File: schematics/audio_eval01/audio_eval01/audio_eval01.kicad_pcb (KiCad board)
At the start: 2 copper layers, 31.1 x 28.6 mm, 2 parts, among them J1 Conn_01x08_Pin

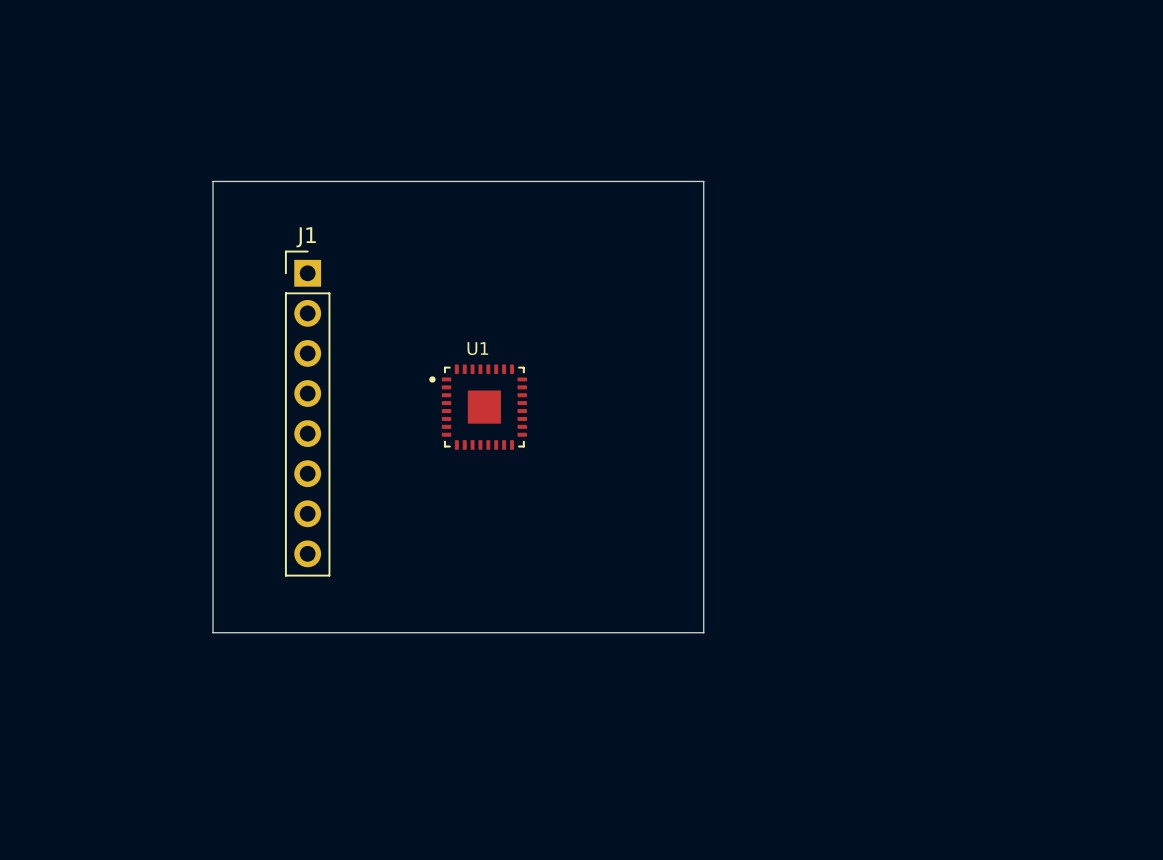
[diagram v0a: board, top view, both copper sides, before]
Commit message: Audio evaluation board work.
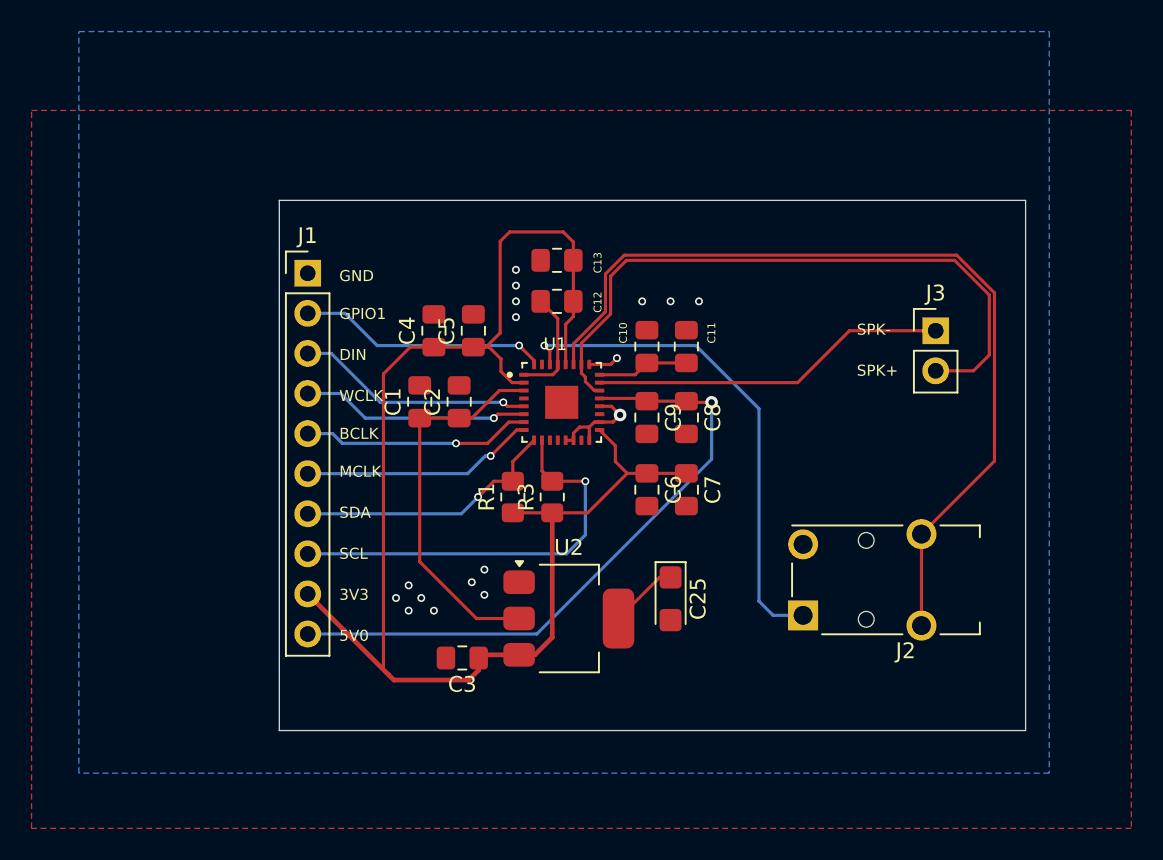
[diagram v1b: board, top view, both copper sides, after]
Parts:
- added C1: 0.1uF, Capacitor_SMD:C_0805_2012Metric_Pad1.18x1.45mm_HandSolder, F.Cu at (136.1, 83.0)
- added C10: 0.1uF, Capacitor_SMD:C_0805_2012Metric_Pad1.18x1.45mm_HandSolder, F.Cu at (150.5, 79.5)
- added C11: 22uF, Capacitor_SMD:C_0805_2012Metric_Pad1.18x1.45mm_HandSolder, F.Cu at (153.0, 79.5)
- added C12: 0.1uF, Capacitor_SMD:C_0805_2012Metric_Pad1.18x1.45mm_HandSolder, F.Cu at (144.8, 76.6)
- added C13: 10uF, Capacitor_SMD:C_0805_2012Metric_Pad1.18x1.45mm_HandSolder, F.Cu at (144.8, 74.0)
- added C2: 10uF, Capacitor_SMD:C_0805_2012Metric_Pad1.18x1.45mm_HandSolder, F.Cu at (138.6, 83.0)
- added C25: 47uF, Capacitor_Tantalum_SMD:CP_EIA-3216-18_Kemet-A, F.Cu at (152.0, 95.4)
- added C3: 10uF, Capacitor_SMD:C_0805_2012Metric_Pad1.18x1.45mm_HandSolder, F.Cu at (138.8, 99.2)
- added C4: 0.1uF, Capacitor_SMD:C_0805_2012Metric_Pad1.18x1.45mm_HandSolder, F.Cu at (137.0, 78.5)
- added C5: 10uF, Capacitor_SMD:C_0805_2012Metric_Pad1.18x1.45mm_HandSolder, F.Cu at (139.5, 78.5)
- added C6: 0.1uF, Capacitor_SMD:C_0805_2012Metric_Pad1.18x1.45mm_HandSolder, F.Cu at (150.5, 88.5)
- added C7: 10uF, Capacitor_SMD:C_0805_2012Metric_Pad1.18x1.45mm_HandSolder, F.Cu at (153.0, 88.5)
- added C8: 0.1uF, Capacitor_SMD:C_0805_2012Metric_Pad1.18x1.45mm_HandSolder, F.Cu at (153.0, 84.0)
- added C9: 22uF, Capacitor_SMD:C_0805_2012Metric_Pad1.18x1.45mm_HandSolder, F.Cu at (150.5, 84.0)
- added J2: AudioJack3, Connector_Audio:Jack_3.5mm_Switronic_ST-005-G_horizontal, F.Cu at (166.9, 94.2)
- added J3: Conn_01x02_Pin, Connector_PinHeader_2.54mm:PinHeader_1x02_P2.54mm_Vertical, F.Cu at (168.8, 78.5)
- added R1: R, Resistor_SMD:R_0805_2012Metric_Pad1.20x1.40mm_HandSolder, F.Cu at (142.0, 89.0)
- added R3: R, Resistor_SMD:R_0805_2012Metric_Pad1.20x1.40mm_HandSolder, F.Cu at (144.5, 89.0)
- added U2: AMS1117-1.8, Package_TO_SOT_SMD:SOT-223-3_TabPin2, F.Cu at (145.6, 96.7)
- J1: value Conn_01x08_Pin -> Conn_01x10_Pin; footprint Connector_PinHeader_2.54mm:PinHeader_1x08_P2.54mm_Vertical -> Connector_PinHeader_2.54mm:PinHeader_1x10_P2.54mm_Vertical
- moved U1 4.91 mm to (145.1, 83.0)
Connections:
- J1 pad 1: WCLK -> GND
- J1 pad 2: BCLK -> GPIO1
- J1 pad 3: MCLK -> DIN
- J1 pad 4: SDA -> WCLK
- J1 pad 5: SCL -> BCLK
- J1 pad 6: unconnected-(J1-Pin_6-Pad6) -> MCLK
- J1 pad 7: unconnected-(J1-Pin_7-Pad7) -> SDA
- J1 pad 8: GPIO1 -> SCL
- U1 pad 13: unconnected-(U1-AIN1-Pad13) -> GND
- U1 pad 14: unconnected-(U1-AIN2-Pad14) -> GND
- U1 pad 17: unconnected-(U1-AVDD-Pad17) -> 3V3
- U1 pad 19: unconnected-(U1-SPKM-Pad19) -> Net-(J3-Pin_1)
- U1 pad 2: unconnected-(U1-IOVDD-Pad2) -> 3V3
- U1 pad 21: unconnected-(U1-SPKVDD-Pad21) -> 5V0
- U1 pad 22: unconnected-(U1-SPKP-Pad22) -> Net-(J3-Pin_2)
- U1 pad 23: unconnected-(U1-SPKM-Pad23) -> Net-(J3-Pin_1)
- U1 pad 24: unconnected-(U1-SPKVDD-Pad24) -> 5V0
- U1 pad 26: unconnected-(U1-SPKP-Pad26) -> Net-(J3-Pin_2)
- U1 pad 27: unconnected-(U1-HPL-Pad27) -> Net-(U1-HPL)
- U1 pad 28: unconnected-(U1-HPVDD-Pad28) -> 3V3
- U1 pad 3: unconnected-(U1-DVDD-Pad3) -> 1V8
- U1 pad 30: unconnected-(U1-HPR-Pad30) -> Net-(U1-HPR)
- U1 pad 5: unconnected-(U1-DIN-Pad5) -> DIN
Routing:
- net 3V3: track 0.00 -> 93.9 mm
- net Net-(U1-HPL): track 0.00 -> 55.7 mm
- net 5V0: track 0.00 -> 46.8 mm, vias 0 -> 1
- net Net-(J3-Pin_2): track 0.00 -> 41.6 mm
- net Net-(U1-HPR): track 0.00 -> 32.0 mm, vias 0 -> 1
- net 1V8: track 0.00 -> 28.6 mm
- net SCL: track 0.00 -> 26.5 mm, vias 0 -> 1
- net Net-(J3-Pin_1): track 0.00 -> 22.7 mm
- net SDA: track 0.00 -> 17.0 mm, vias 0 -> 1
- net GPIO1: track 0.00 -> 15.8 mm, vias 0 -> 1
- net GND: track 0.00 -> 15.7 mm, vias 0 -> 17
- net DIN: track 0.00 -> 15.1 mm, vias 0 -> 1
- net MCLK: track 0.00 -> 14.8 mm, vias 0 -> 1
- net BCLK: track 0.00 -> 14.5 mm, vias 0 -> 1
- net WCLK: track 0.00 -> 14.4 mm, vias 0 -> 1
- added copper zone on B.Cu, net GND
- added copper zone on F.Cu, net GND
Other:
- board size 31.1 x 28.6 mm -> 47.3 x 33.6 mm
- board text added: "3V3"
- board text added: "5V0"
- board text added: "BCLK"
- board text added: "DIN"
- board text added: "GND"
- board text added: "GPIO1"
- board text added: "MCLK"
- board text added: "SCL"
- board text added: "SDA"
- board text added: "SPK+"
- board text added: "SPK-"
- board text added: "WCLK"
